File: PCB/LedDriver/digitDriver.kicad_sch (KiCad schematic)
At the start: 43 parts, among them U201 NJW4617DL3-TE1, U202 NJW4617DL3-TE1, U203 NJW4617DL3-TE1, U204 NJW4617DL3-TE1, U205 NJW4617DL3-TE1, U206 NJW4617DL3-TE1, U207 NJW4617DL3-TE1, U208 74HC595

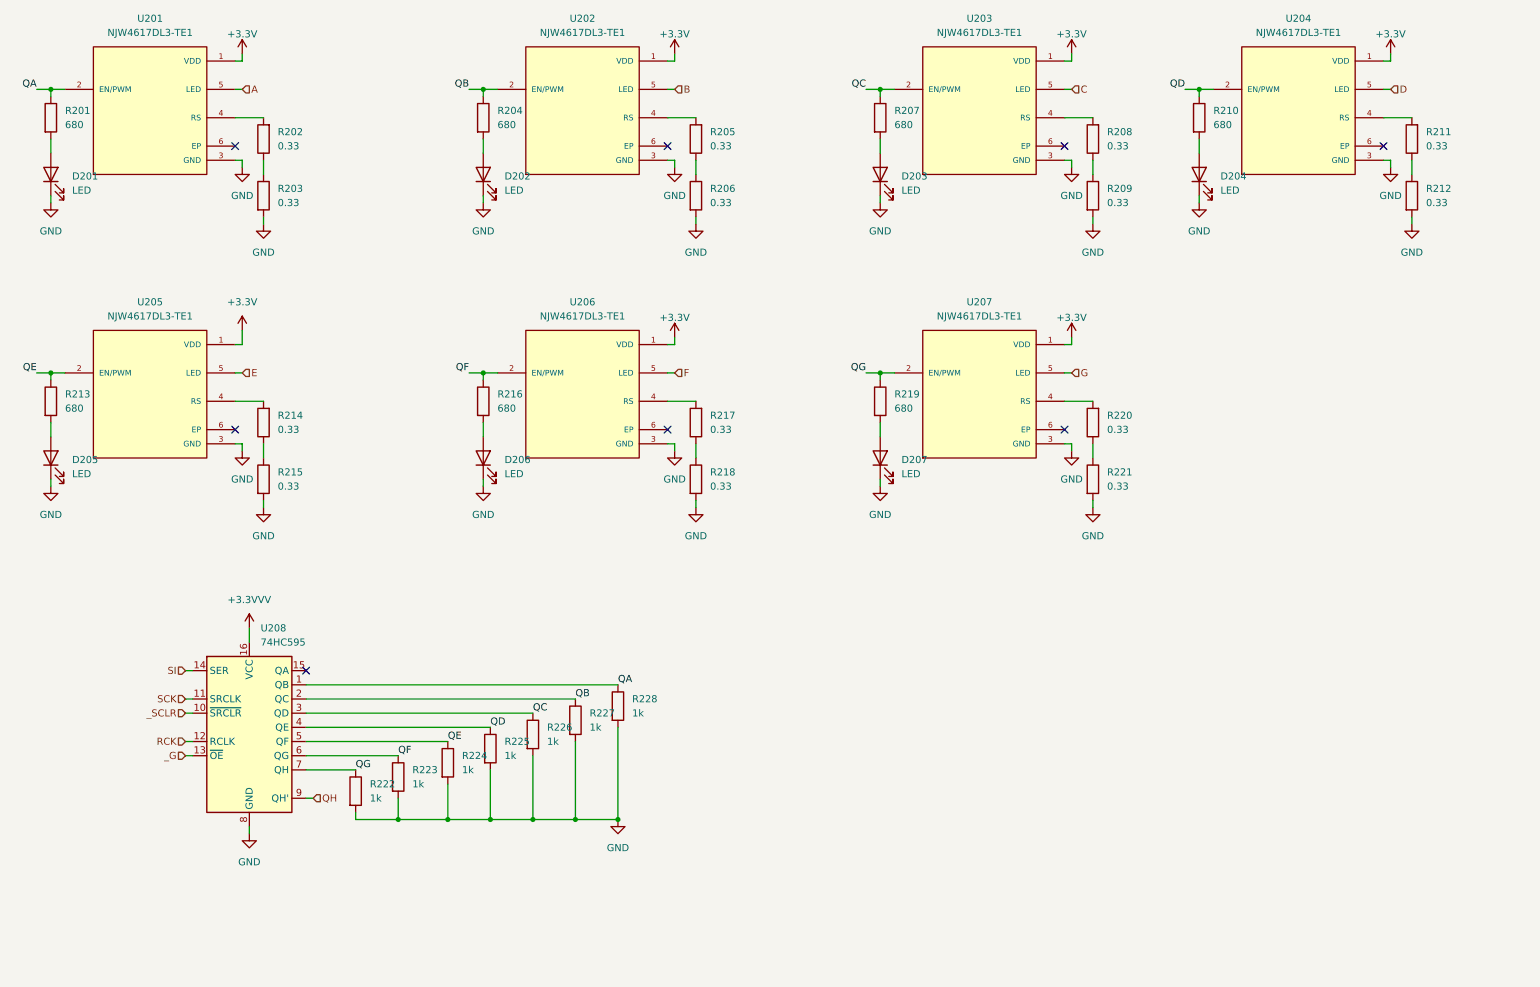
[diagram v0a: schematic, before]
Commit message: 基板改良
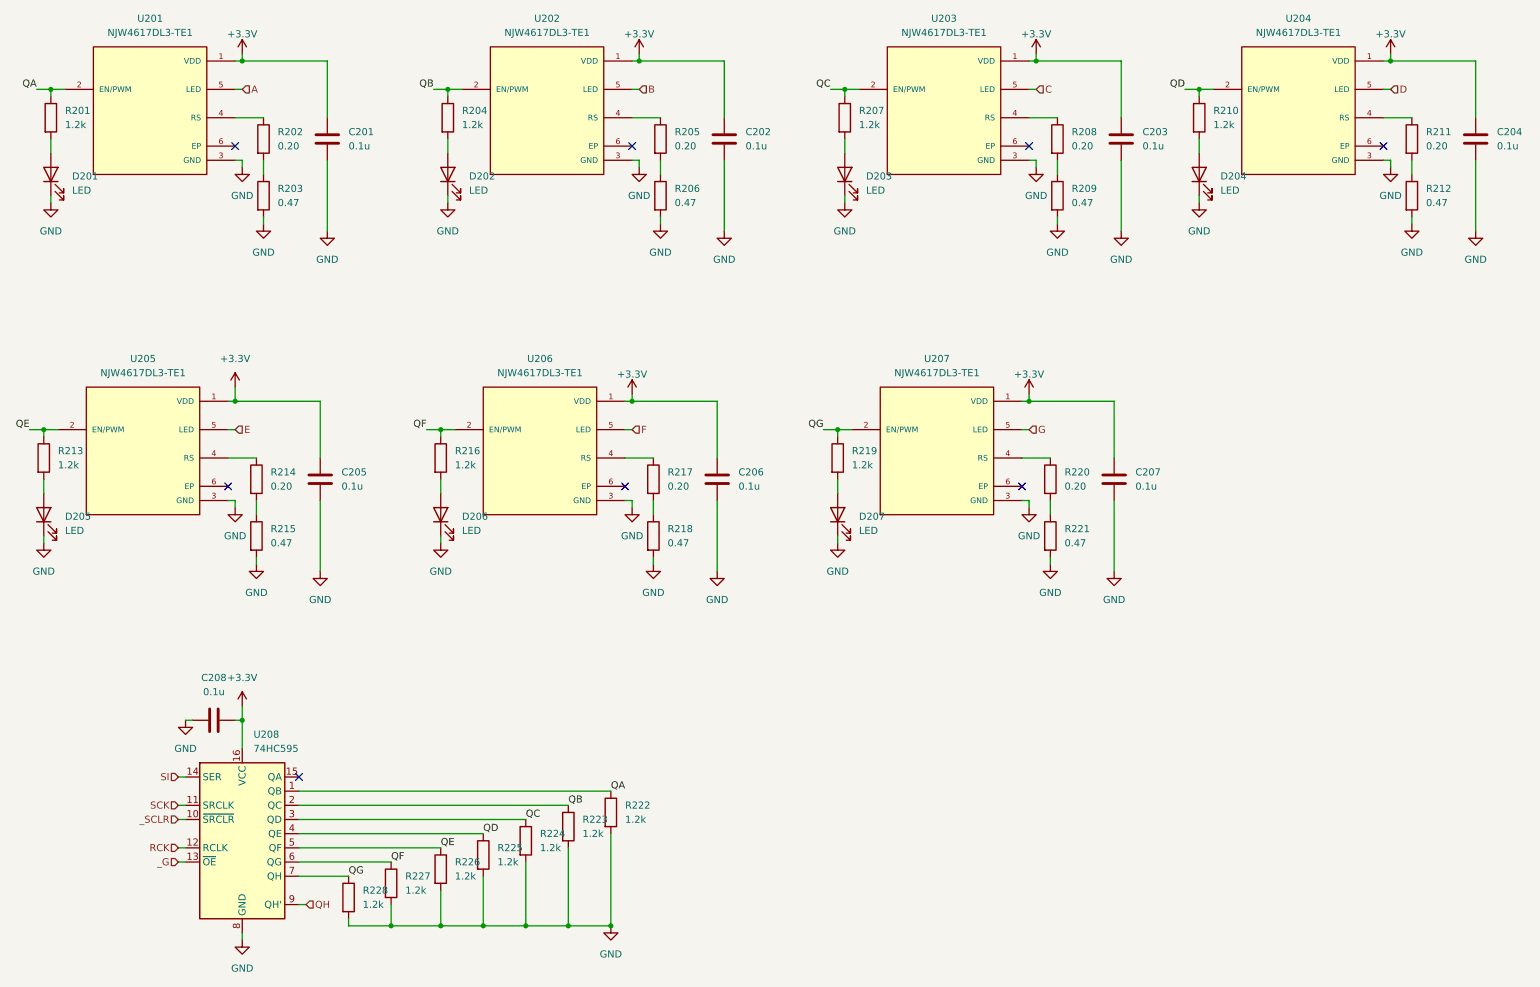
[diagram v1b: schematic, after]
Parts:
- removed R228: 1k, Resistor_SMD:R_0603_1608Metric, symbol Device:R
- added C201, C202, C203, C204, C205, C206, C207, C208: 0.1u, Capacitor_SMD:C_0603_1608Metric, symbol Device:C
- added R222: 1.2k, Resistor_SMD:R_0603_1608Metric, symbol Device:R
- R201, R204, R207, R210, R213, R216, R219: value 680 -> 1.2k
- R202, R205, R208, R211, R214, R217, R220: value 0.33 -> 0.20; footprint Resistor_THT:R_Axial_DIN0207_L6.3mm_D2.5mm_P7.62mm_Horizontal -> Resistor_THT:R_Axial_DIN0207_L6.3mm_D2.5mm_P10.16mm_Horizontal
- R203, R206, R209, R212, R215, R218, R221: value 0.33 -> 0.47; footprint Resistor_THT:R_Axial_DIN0207_L6.3mm_D2.5mm_P7.62mm_Horizontal -> Resistor_THT:R_Axial_DIN0207_L6.3mm_D2.5mm_P10.16mm_Horizontal
- R223, R224, R225, R226, R227: value 1k -> 1.2k
- R228: renamed from R222; value 1k -> 1.2k
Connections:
- net +3.3V: now also C201.1, C202.1, C203.1, C204.1, C205.1, C206.1, C207.1, C208.2
- net GND: now also C201.2, C202.2, C203.2, C204.2, C205.2, C206.2, C207.2, C208.1, R222.2
- net QA: now also R222.1
- net QB: now also R223.1; no longer R227.1
- net QC: now also R224.1; no longer R226.1
- net QE: now also R226.1; no longer R224.1
- net QF: now also R227.1; no longer R223.1
- net at R214.1: now also U205.4 (RS); no longer R215.1
- net at R214.2: now also R215.1; no longer U205.4 (RS)
- net at U207.4 (RS): now also R220.1; no longer R220.2
- net at R211.2: now also R212.1; no longer U204.4 (RS)
- net at R206.1: now also R205.2; no longer R205.1
- net at U202.4 (RS): now also R205.1; no longer R205.2
- net at R202.2: now also R203.1; no longer U201.4 (RS)
- net at R218.1: now also R217.2; no longer R217.1
- net at U206.4 (RS): now also R217.1; no longer R217.2
- net at R209.1: now also R208.2; no longer R208.1
- net at U203.4 (RS): now also R208.1; no longer R208.2
- net at R202.1: now also U201.4 (RS); no longer R203.1
- net at R221.1: now also R220.2; no longer R220.1
- net at R211.1: now also U204.4 (RS); no longer R212.1
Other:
- moved on the sheet: D202, D203, D205, D206, D207, R204, R228, U202, U203, U205, U206, U207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
